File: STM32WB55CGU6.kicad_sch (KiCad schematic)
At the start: 25 parts, among them IC2 STM32WB55CGU6, J11 BOOT0_Jumper, Y1 ABM3B-32.000MHZ-8-R30-B1U-T

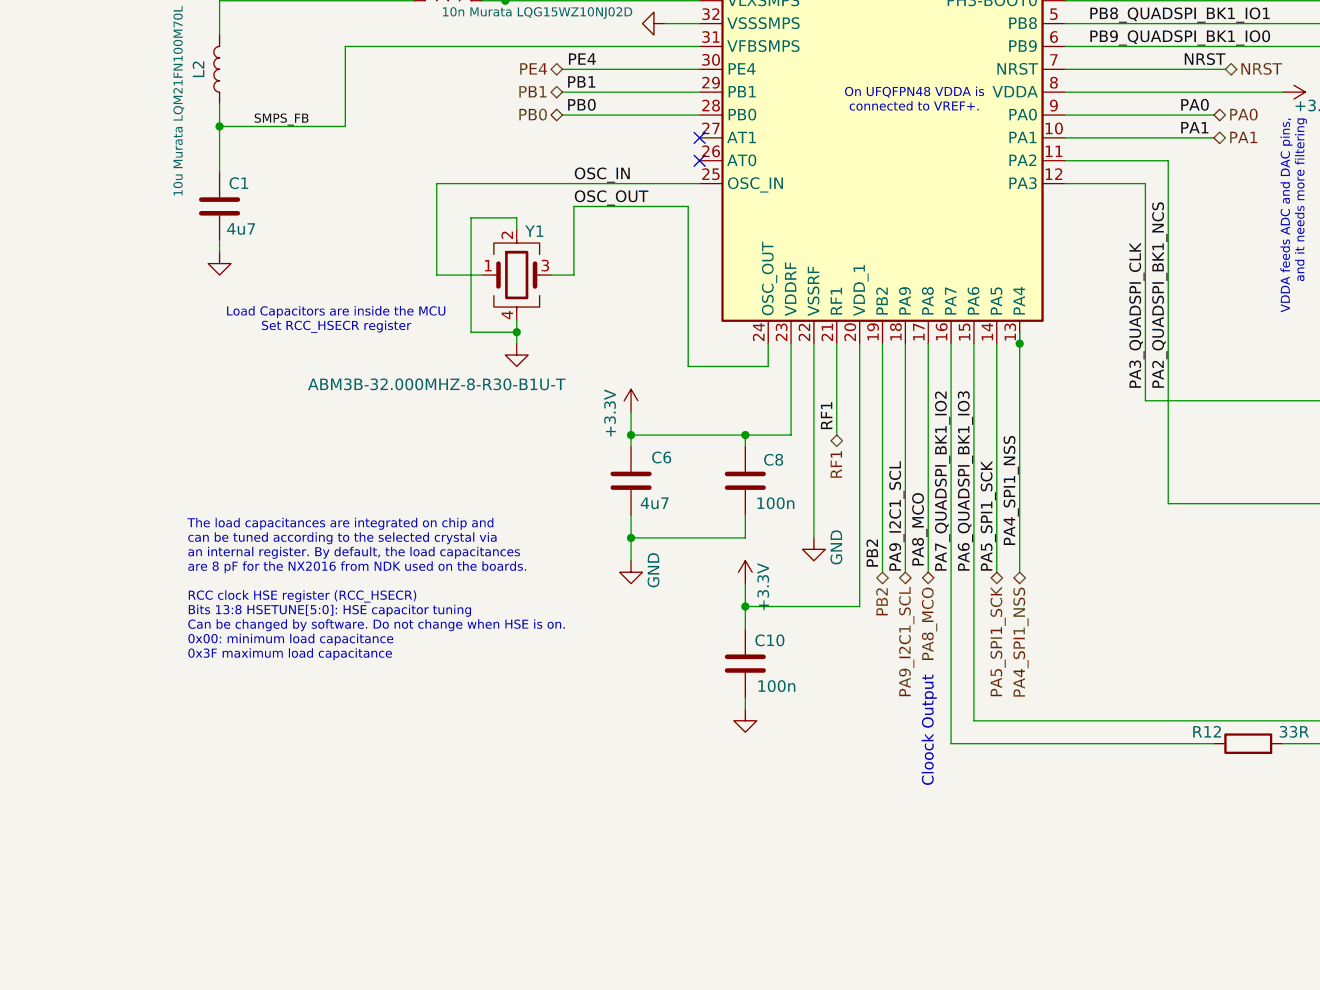
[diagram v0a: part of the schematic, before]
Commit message: Update
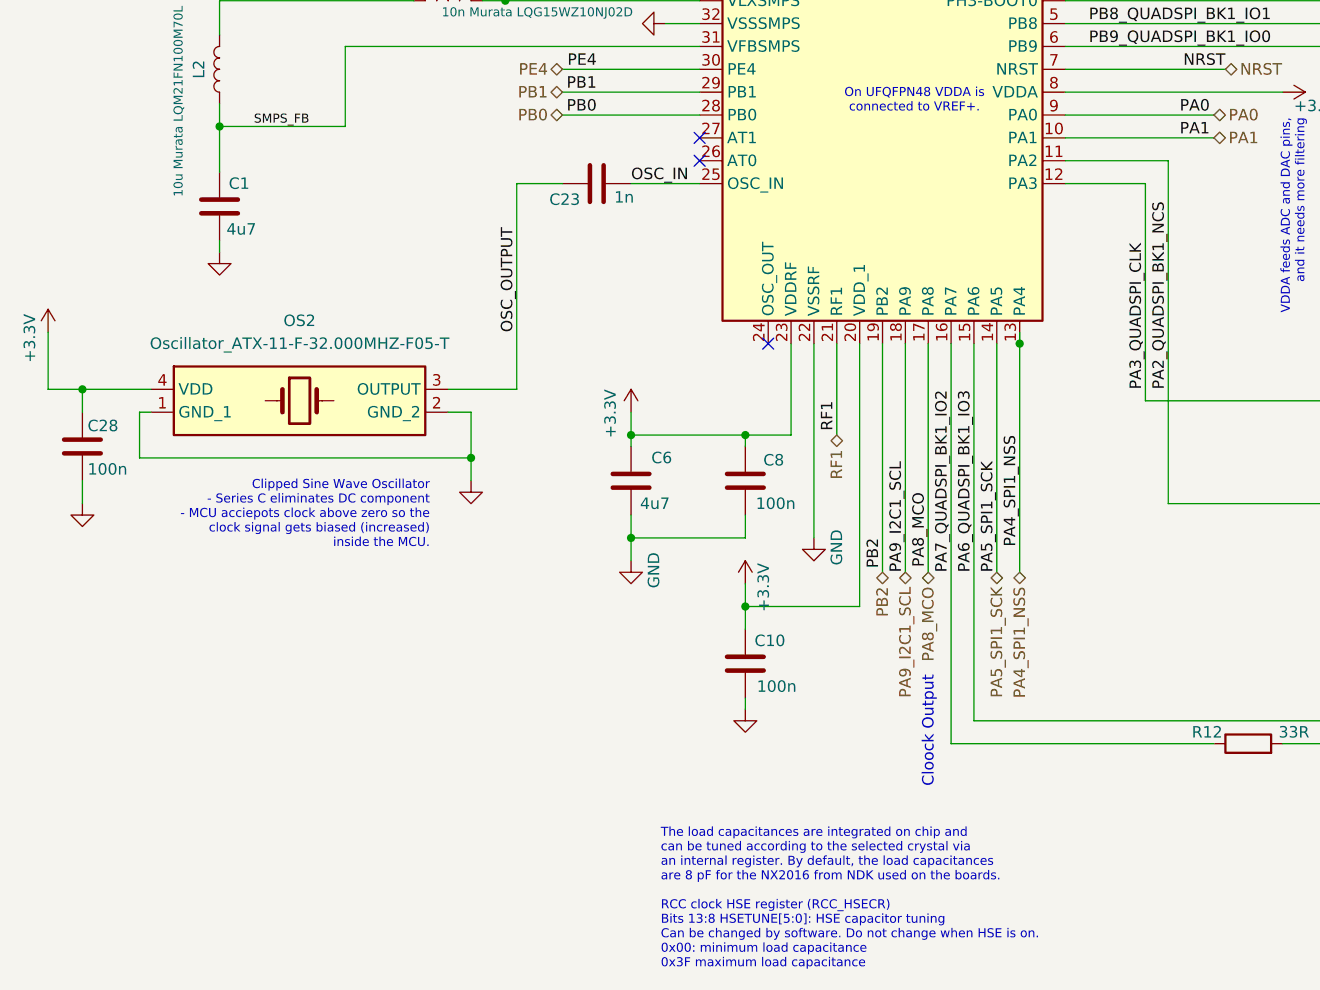
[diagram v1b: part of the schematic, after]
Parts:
- removed Y1: ABM3B-32.000MHZ-8-R30-B1U-T, Personal_Project:XTAL_ABM3B-32.000MHZ-10-R30-B1U-T, symbol Personal_Projects:ABM3B-32.000MHZ-10-R30-B1U-T
- added C23: 1n, Capacitor_SMD:C_0805_2012Metric, symbol Device:C
- added C28: 100n, Capacitor_SMD:C_0805_2012Metric, symbol Device:C
- added OS2: Oscillator_ATX-11-F-32.000MHZ-F05-T, Personal_Project:Oscillator_ECSTXO32CSMV320ANTR, symbol Personal_Projects:Oscillator_ECS-TXO-32CSMV-320-AN-TR
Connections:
- net +3.3V: now also C28.2, OS2.4 (VDD)
- net GND: now also C28.1, OS2.1 (GND_1), OS2.2 (GND_2)
- net OSC_IN: now also C23.1
- net OSC_OUT: no longer names the net of IC2.24 (OSC_OUT)
- new net OSC_OUTPUT: C23.2, OS2.3 (OUTPUT)
- no-connect marks 4 -> 5
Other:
- note added: "Clipped Sine Wave Oscillator - Series C eliminates DC component - MCU acciepots clock above zero so the clock signal gets biased (increased) inside the MCU."
- note removed: "Load Capacitors are inside the MCU Set RCC_HSECR register"
